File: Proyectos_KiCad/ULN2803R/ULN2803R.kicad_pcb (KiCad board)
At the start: 2 copper layers, 50 x 45 mm, 9 parts, among them J1 IN, J2 OUT, J3 CARGADOR, J4 RELES, U1 ULN2803A

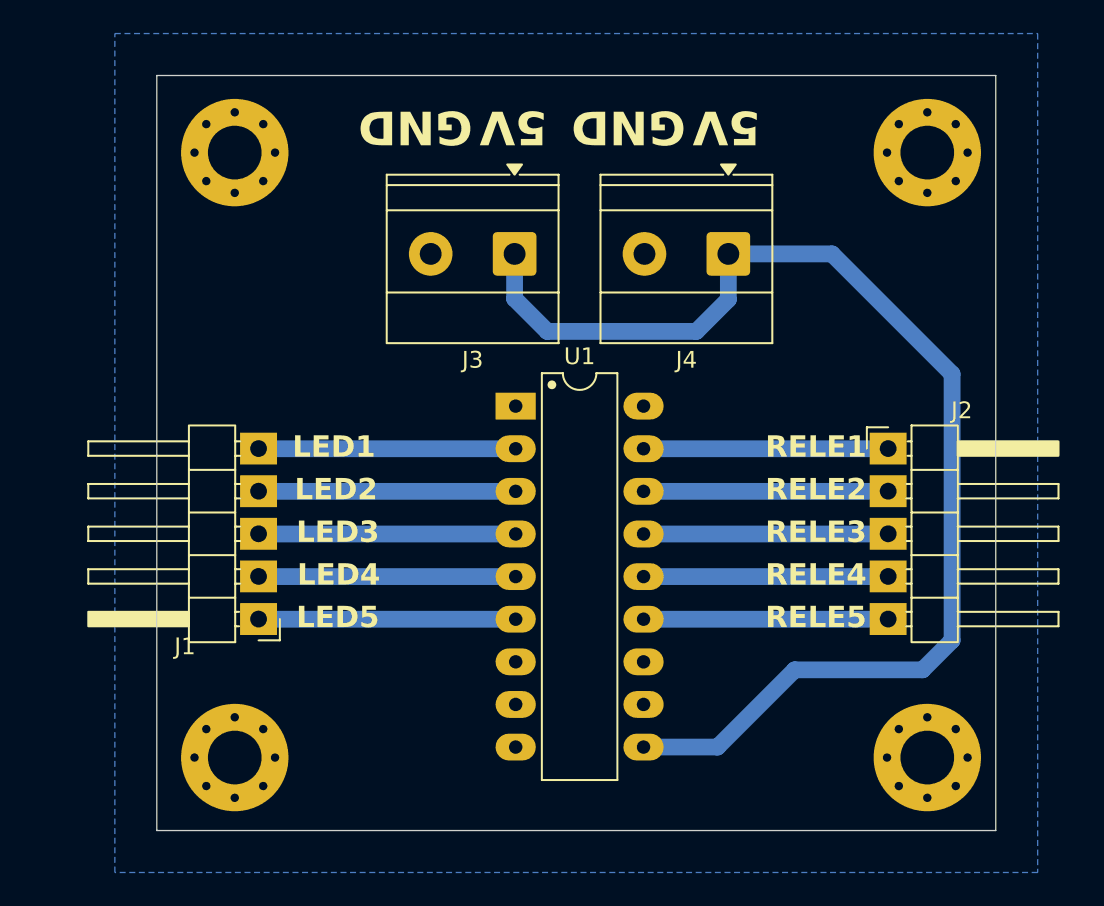
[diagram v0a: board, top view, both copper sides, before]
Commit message: Shiel-ULN2803-BPM
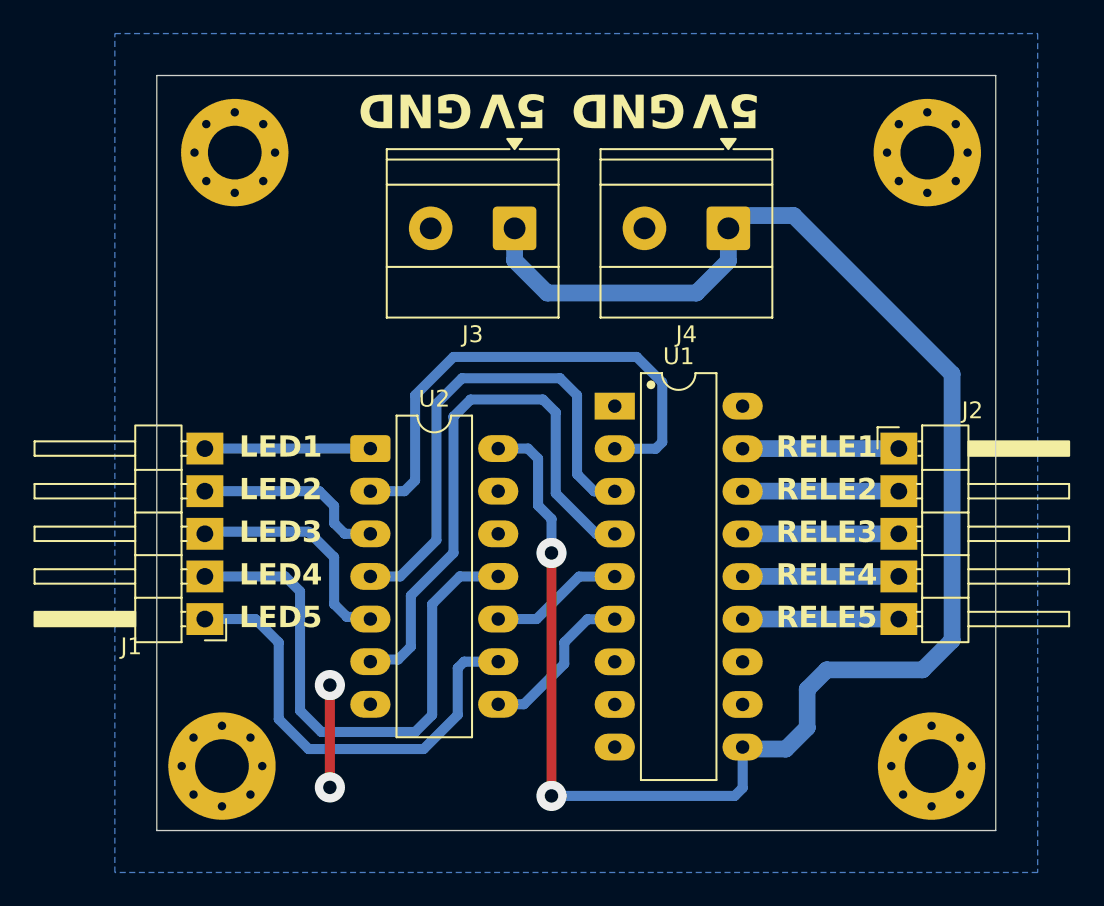
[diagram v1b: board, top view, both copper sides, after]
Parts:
- added U2: 74LS14, Package_DIP:CERDIP-14_W7.62mm_SideBrazed_LongPads, F.Cu at (117.7, 102.2)
- moved U1 5.90 mm to (132.3, 99.7)
- moved J1 3.20 mm to (107.9, 112.4)
- moved J3 1.52 mm to (126.3, 89.1)
- moved J4 1.52 mm to (139.1, 89.1)
- moved H4 0.92 mm to (108.9, 121.2)
- moved J2 0.63 mm to (149.2, 102.2)
- moved H3 0.57 mm to (151.2, 121.2)
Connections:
- U1 pad 2: Net-(J1-Pin_5) -> Net-(U1-I2)
- U1 pad 3: Net-(J1-Pin_4) -> Net-(U1-I3)
- U1 pad 4: Net-(J1-Pin_3) -> Net-(U1-I4)
- U1 pad 5: Net-(J1-Pin_2) -> Net-(U1-I5)
- U1 pad 6: Net-(J1-Pin_1) -> Net-(U1-I6)
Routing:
- net Net-(U1-I4): track 0.00 -> 33.7 mm
- net VCC: track 72.9 -> 106.5 mm, vias 0 -> 2
- net Net-(U1-I2): track 0.00 -> 30.9 mm
- net Net-(U1-I3): track 0.00 -> 29.8 mm
- net Net-(J1-Pin_2): track 15.3 -> 33.2 mm
- net Net-(J1-Pin_1): track 15.3 -> 27.2 mm
- net Net-(U1-I6): track 0.00 -> 9.79 mm
- net Net-(U1-I5): track 0.00 -> 7.99 mm
- net GND: track 0.00 -> 6.10 mm, vias 0 -> 2
- net Net-(J1-Pin_5): track 15.3 -> 9.86 mm
- net Net-(J2-Pin_4): track 14.6 -> 9.33 mm
- net Net-(J2-Pin_5): track 14.6 -> 9.33 mm
- net Net-(J2-Pin_3): track 14.6 -> 9.33 mm
- net Net-(J2-Pin_1): track 14.6 -> 9.33 mm
- net Net-(J2-Pin_2): track 14.6 -> 9.96 mm
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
